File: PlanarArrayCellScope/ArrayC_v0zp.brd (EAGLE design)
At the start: 41.1 x 41.1 mm, 121 parts

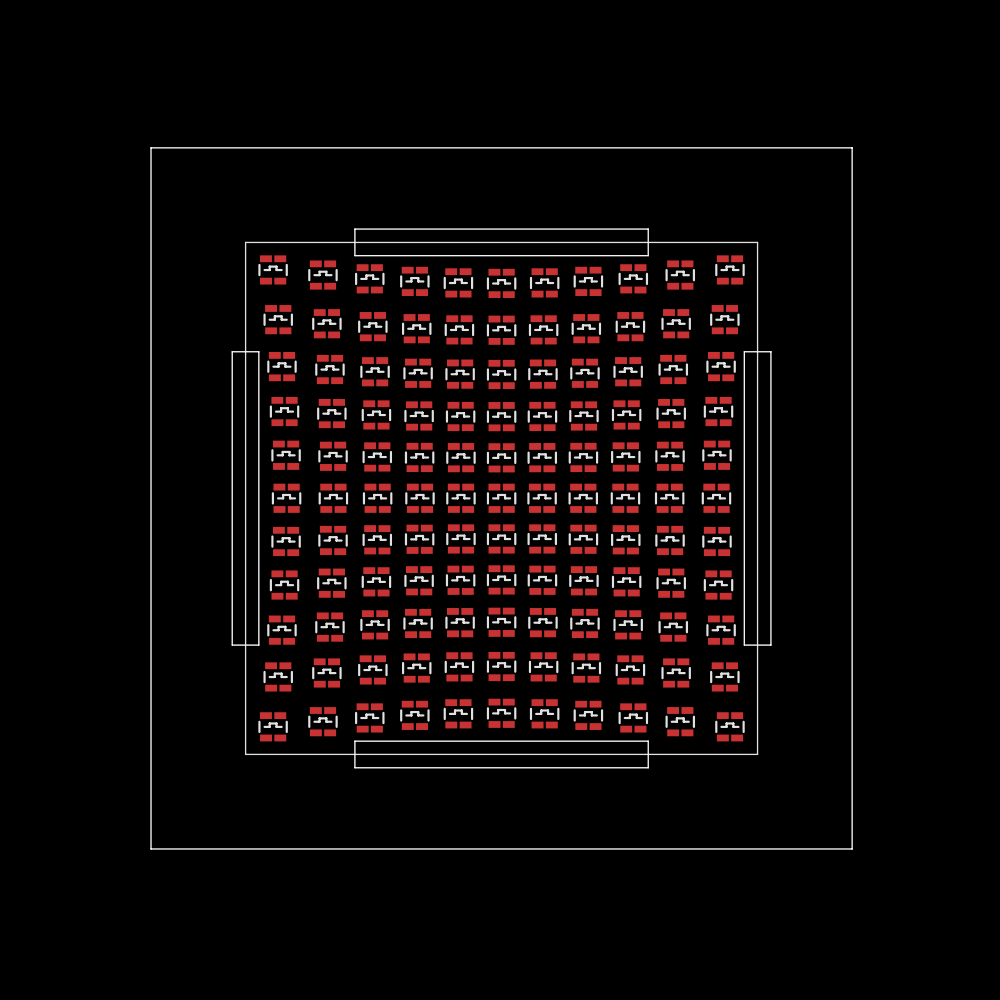
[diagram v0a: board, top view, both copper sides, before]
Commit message: Updated Planar Array Designs
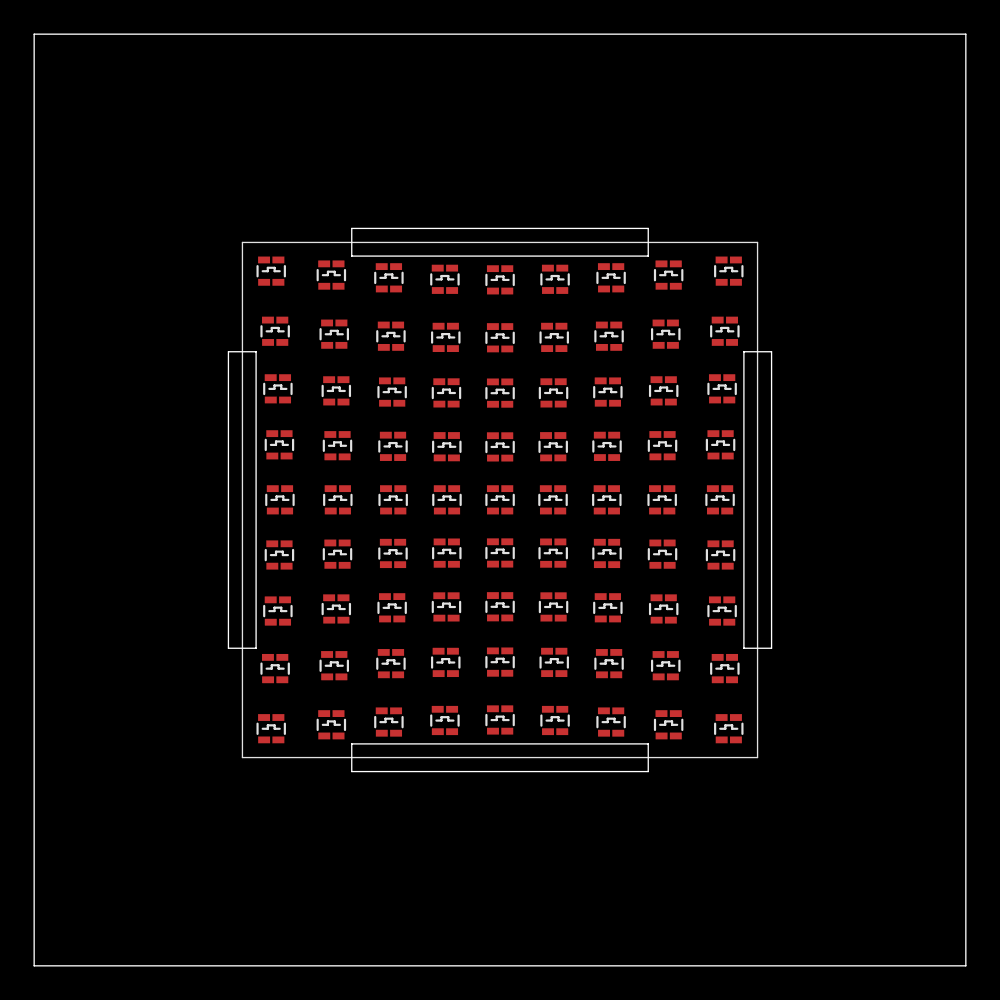
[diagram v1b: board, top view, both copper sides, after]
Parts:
- removed LED100, LED101, LED102, LED103, LED104, LED105, LED106, LED107, LED108, LED109, LED110, LED111, LED112, LED113, LED114, LED115, LED116, LED117, LED118, LED119, LED120, LED81, LED82, LED83, LED84, LED85, LED86, LED87, LED88, LED89, LED90, LED91, LED92, LED93, LED94, LED95, LED96, LED97, LED98, LED99: KB_APTF1616V0, ZacksLib:KB_RGBLED_APTF1616
- LED00, LED01, LED02, LED03, LED04, LED05, LED06, LED07, LED08, LED09, LED10, LED11, LED12, LED13, LED14, LED15, LED16, LED17, LED18, LED19, LED20, LED21, LED22, LED23, LED24, LED25, LED26, LED27, LED28, LED29, LED30, LED31, LED32, LED33, LED34, LED35, LED36, LED37, LED38, LED39, LED40, LED41, LED42, LED43, LED44, LED45, LED46, LED47, LED48, LED49, LED50, LED51, LED52, LED53, LED54, LED55, LED56, LED57, LED58, LED59, LED60, LED61, LED62, LED63, LED64, LED65, LED66, LED67, LED68, LED69, LED70, LED71, LED72, LED73, LED74, LED75, LED76, LED77, LED78, LED79, LED80: device ZacksLib:KB_RGBLED_APTF1616 -> WallerLabLib:KB_RGBLED_APTF1616
- moved LED54 27.2 mm to (33.8, 14.3)
- moved LED44 25.5 mm to (27.3, 40.2)
- moved LED09 23.9 mm to (17.4, 14.1)
- moved LED10 23.4 mm to (17.6, 17.6)
- moved LED63 22.7 mm to (37.1, 14.1)
- moved LED64 21.9 mm to (37.0, 17.6)
- moved LED65 21.3 mm to (36.9, 20.9)
- moved LED35 20.2 mm to (24.1, 40.2)
- moved LED80 20.0 mm to (40.7, 40.7)
- moved LED34 19.4 mm to (24.1, 36.8)
- moved LED72 19.3 mm to (40.7, 13.9)
- moved LED33 19.0 mm to (24.1, 33.5)
- moved LED79 19.0 mm to (40.4, 37.1)
- moved LED18 18.4 mm to (20.8, 14.3)
- moved LED73 18.2 mm to (40.4, 17.4)
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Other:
- board size 41.1 x 41.1 mm -> 54.6 x 54.6 mm
